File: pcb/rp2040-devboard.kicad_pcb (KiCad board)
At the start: 2 copper layers, 0 parts

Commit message: wip pcb placement
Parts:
- added C301: 1u, Capacitor_SMD:C_1210_3225Metric_Pad1.33x2.70mm_HandSolder, F.Cu at (98.0, 99.3)
- added C302: 1u, Capacitor_SMD:C_1210_3225Metric_Pad1.33x2.70mm_HandSolder, F.Cu at (98.0, 103.6)
- added C401: TBD, Capacitor_SMD:C_1210_3225Metric_Pad1.33x2.70mm_HandSolder, F.Cu at (98.0, 53.5)
- added C402: 100n, Capacitor_SMD:C_1210_3225Metric_Pad1.33x2.70mm_HandSolder, F.Cu at (98.0, 57.8)
- added C403: 100n, Capacitor_SMD:C_1210_3225Metric_Pad1.33x2.70mm_HandSolder, F.Cu at (98.0, 62.0)
- added C404: 1u, Capacitor_SMD:C_1210_3225Metric_Pad1.33x2.70mm_HandSolder, F.Cu at (98.0, 66.3)
- added C405: 100n, Capacitor_SMD:C_1210_3225Metric_Pad1.33x2.70mm_HandSolder, F.Cu at (98.0, 70.5)
- added C406: 100n, Capacitor_SMD:C_1210_3225Metric_Pad1.33x2.70mm_HandSolder, F.Cu at (104.0, 53.5)
- added C407: 100n, Capacitor_SMD:C_1210_3225Metric_Pad1.33x2.70mm_HandSolder, F.Cu at (104.0, 57.8)
- added C408: 100n, Capacitor_SMD:C_1210_3225Metric_Pad1.33x2.70mm_HandSolder, F.Cu at (104.0, 62.0)
- added C409: 100n, Capacitor_SMD:C_1210_3225Metric_Pad1.33x2.70mm_HandSolder, F.Cu at (104.0, 66.3)
- added C410: 100n, Capacitor_SMD:C_1210_3225Metric_Pad1.33x2.70mm_HandSolder, F.Cu at (104.0, 70.5)
- added C411: 100n, Capacitor_SMD:C_1210_3225Metric_Pad1.33x2.70mm_HandSolder, F.Cu at (110.0, 53.5)
- added C412: 1u, Capacitor_SMD:C_1210_3225Metric_Pad1.33x2.70mm_HandSolder, F.Cu at (110.0, 57.8)
- added C413: 15p, Capacitor_SMD:C_1210_3225Metric_Pad1.33x2.70mm_HandSolder, F.Cu at (110.0, 62.0)
- added C414: 15p, Capacitor_SMD:C_1210_3225Metric_Pad1.33x2.70mm_HandSolder, F.Cu at (110.0, 66.3)
- added C501: 100n, Capacitor_SMD:C_1210_3225Metric_Pad1.33x2.70mm_HandSolder, F.Cu at (128.0, 91.3)
- added D201: ESD441, rp2040-devboard:Texas_X2SON-DPL-2, F.Cu at (111.2, 91.4)
- added D202: ESD321, Diode_SMD:D_SOD-523, F.Cu at (108.5, 91.5)
- added D203: ESD321, Diode_SMD:D_SOD-523, F.Cu at (108.5, 94.0)
- added J201: USB_C_Receptacle_USB2.0_16P, Connector_USB:USB_C_Receptacle_GCT_USB4105-xx-A_16P_TopMnt_Horizontal, F.Cu at (156.0, 51.5)
- added J601: Conn_01x20, Connector_PinHeader_2.54mm:PinHeader_1x20_P2.54mm_Vertical, F.Cu at (141.5, 55.3)
- added J602: Conn_01x20, Connector_PinHeader_2.54mm:PinHeader_1x20_P2.54mm_Vertical, F.Cu at (170.8, 55.2)
- added J603: Conn_01x03, Connector_PinHeader_2.54mm:PinHeader_1x03_P2.54mm_Vertical, F.Cu at (153.7, 105.8)
- added R201: 5.1k 10%, Resistor_SMD:R_1210_3225Metric_Pad1.30x2.65mm_HandSolder, F.Cu at (109.7, 84.0)
- added R202: 5.1k 10%, Resistor_SMD:R_1210_3225Metric_Pad1.30x2.65mm_HandSolder, F.Cu at (109.7, 88.2)
- added R401: TBD, Resistor_SMD:R_1210_3225Metric_Pad1.30x2.65mm_HandSolder, F.Cu at (157.0, 86.2)
- added R402: 27R, Resistor_SMD:R_1210_3225Metric_Pad1.30x2.65mm_HandSolder, F.Cu at (116.0, 57.7)
- added R403: 27R, Resistor_SMD:R_1210_3225Metric_Pad1.30x2.65mm_HandSolder, F.Cu at (116.0, 61.9)
- added R501: TBD, Resistor_SMD:R_1210_3225Metric_Pad1.30x2.65mm_HandSolder, F.Cu at (128.0, 95.5)
- added SW401: SW_Push, rp2040-devboard:SW_SPST_EVPBV, F.Cu at (93.4, 83.5)
- added SW501: SW_Push, rp2040-devboard:SW_SPST_EVPBV, F.Cu at (162.2, 63.9)
- added U301: TC1017-xLT, Package_TO_SOT_SMD:SOT-353_SC-70-5, F.Cu at (103.1, 99.2)
- added U401: RP2040, Package_DFN_QFN:QFN-56-1EP_7x7mm_P0.4mm_EP3.2x3.2mm, F.Cu at (155.3, 74.6)
- added U501: W25Q128JVS, Package_SO:SOIC-8_5.23x5.23mm_P1.27mm, F.Cu at (150.9, 62.4)
- added Y401: ABM8-272-T3, Crystal:Crystal_SMD_3225-4Pin_3.2x2.5mm, F.Cu at (150.7, 86.1)
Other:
- board outline added: 34 x 59 mm

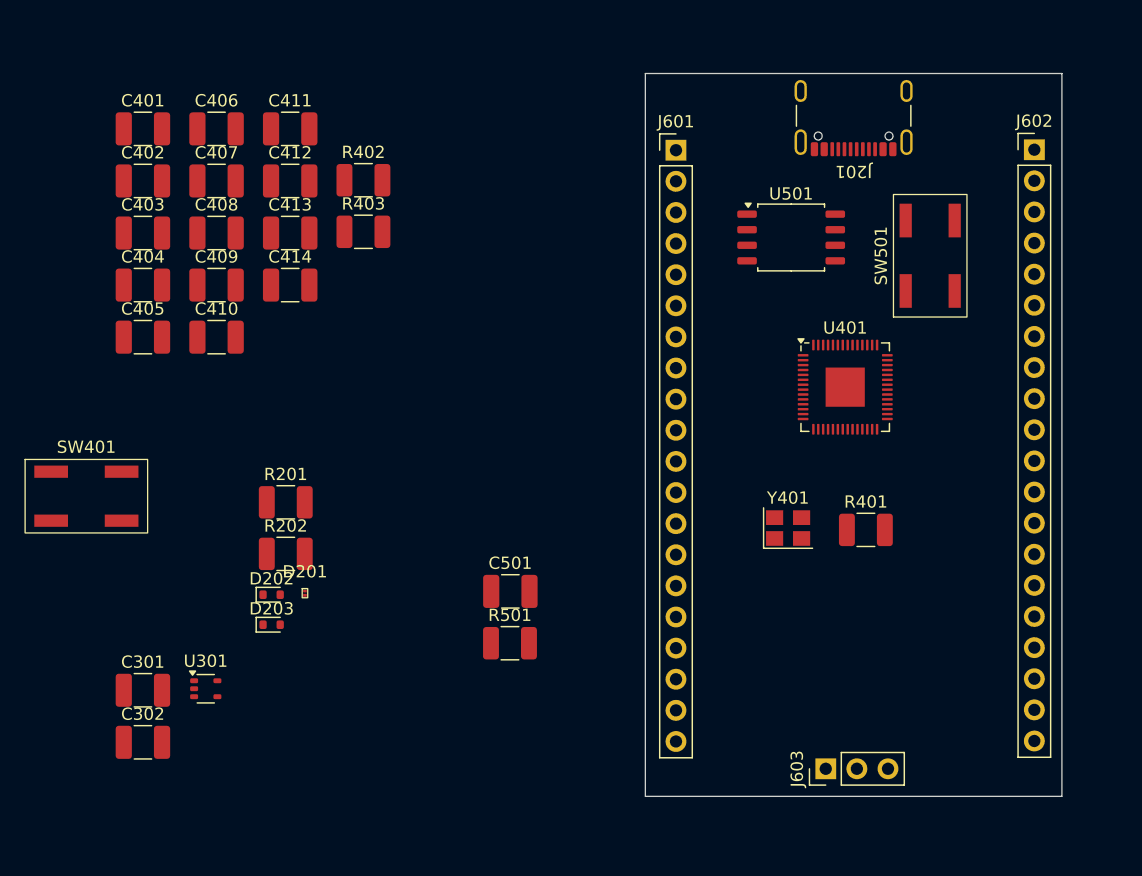
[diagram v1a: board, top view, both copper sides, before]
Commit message: wip pcb placement
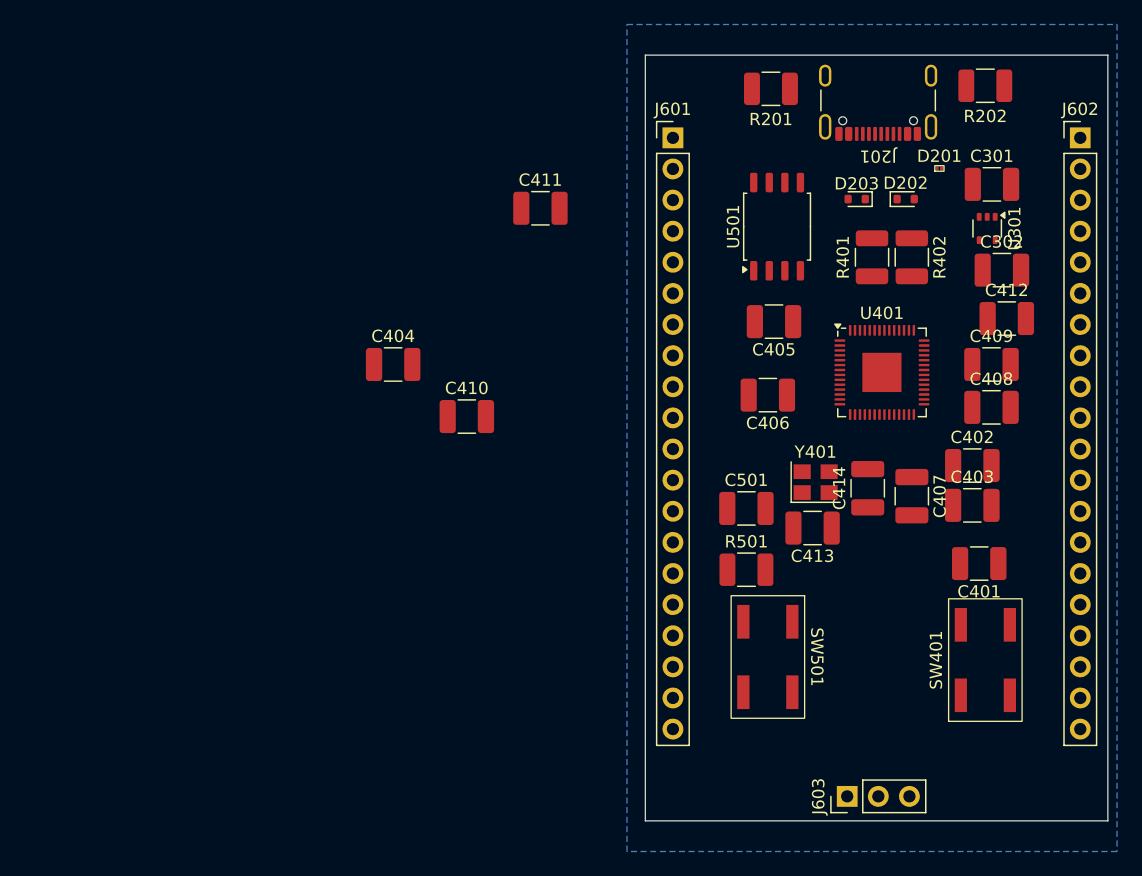
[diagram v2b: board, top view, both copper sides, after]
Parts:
- removed the R401 at (157.0, 86.2)
- moved C301 80.7 mm to (167.3, 58.0)
- moved C302 80.0 mm to (168.1, 65.0)
- moved C401 76.9 mm to (166.2, 89.0), turned to 180 degrees
- moved SW401 74.6 mm to (166.8, 96.9), turned to 90 degrees
- moved U301 74.0 mm to (166.9, 61.6), turned to -90 degrees
- moved C402 71.6 mm to (165.7, 81.0)
- moved C403 71.3 mm to (165.7, 84.2)
- moved R202 68.7 mm to (166.8, 50.0)
- moved C408 64.8 mm to (167.2, 76.2)
- moved C409 63.6 mm to (167.2, 72.8)
- moved D201 62.3 mm to (163.0, 56.8), turned to 90 degrees
- moved C407 62.3 mm to (160.8, 83.5), turned to -90 degrees
- moved D202 61.0 mm to (160.2, 59.2)
- moved C412 59.6 mm to (168.5, 69.0)
- moved D203 59.1 mm to (156.2, 59.2), turned to 180 degrees
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- renumbered R402 to R401, R403 to R402
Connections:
- J602 pad 4: /IO/GPIO26_ADC0 -> /IO/GPIO29_ADC3
- J602 pad 5: /IO/GPIO27_ADC1 -> /IO/GPIO28_ADC2
- J602 pad 6: /IO/GPIO28_ADC2 -> /IO/GPIO27_ADC1
- J602 pad 7: /IO/GPIO29_ADC3 -> /IO/GPIO26_ADC0
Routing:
- added copper zone on B.Cu, net GND
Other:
- board size 34 x 59 mm -> 37.8 x 62.5 mm
